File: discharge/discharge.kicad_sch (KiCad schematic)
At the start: 8 parts, among them J1 Conn_SDC, J2 Conn_HV_IN, J3 Conn_HV_OUT, J4 GND, J5 Conn_HV_IN, J6 Conn_HV_OUT, K1 Relay_SPST-NC, K2 Relay_SPST-NC

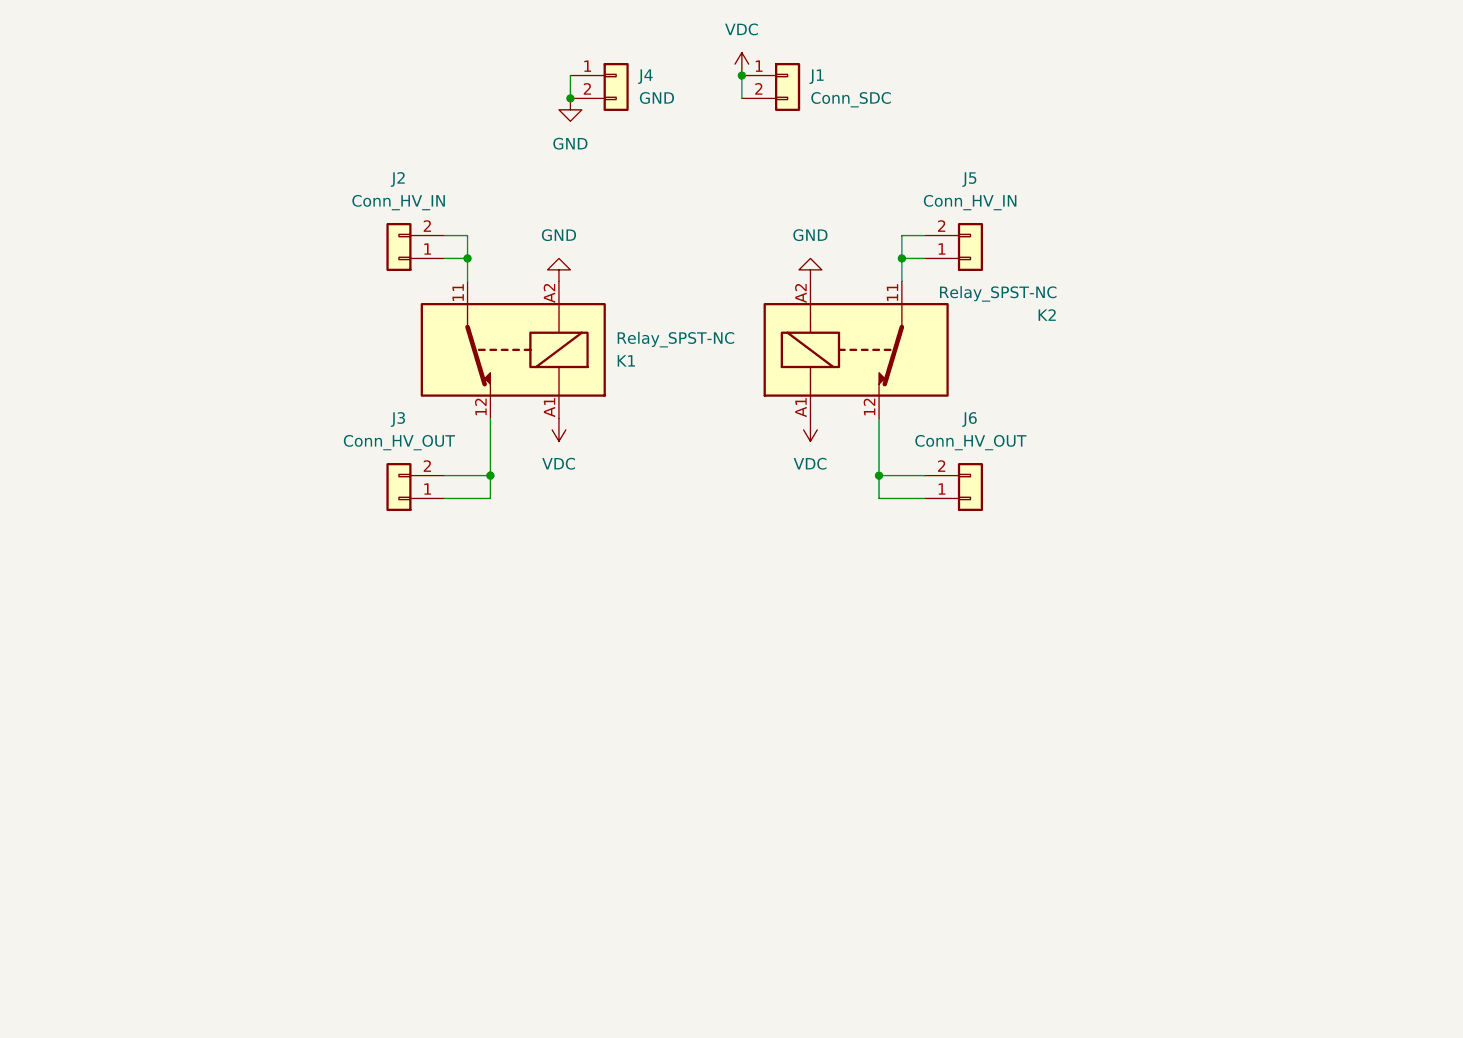
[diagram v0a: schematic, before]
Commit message: add timer
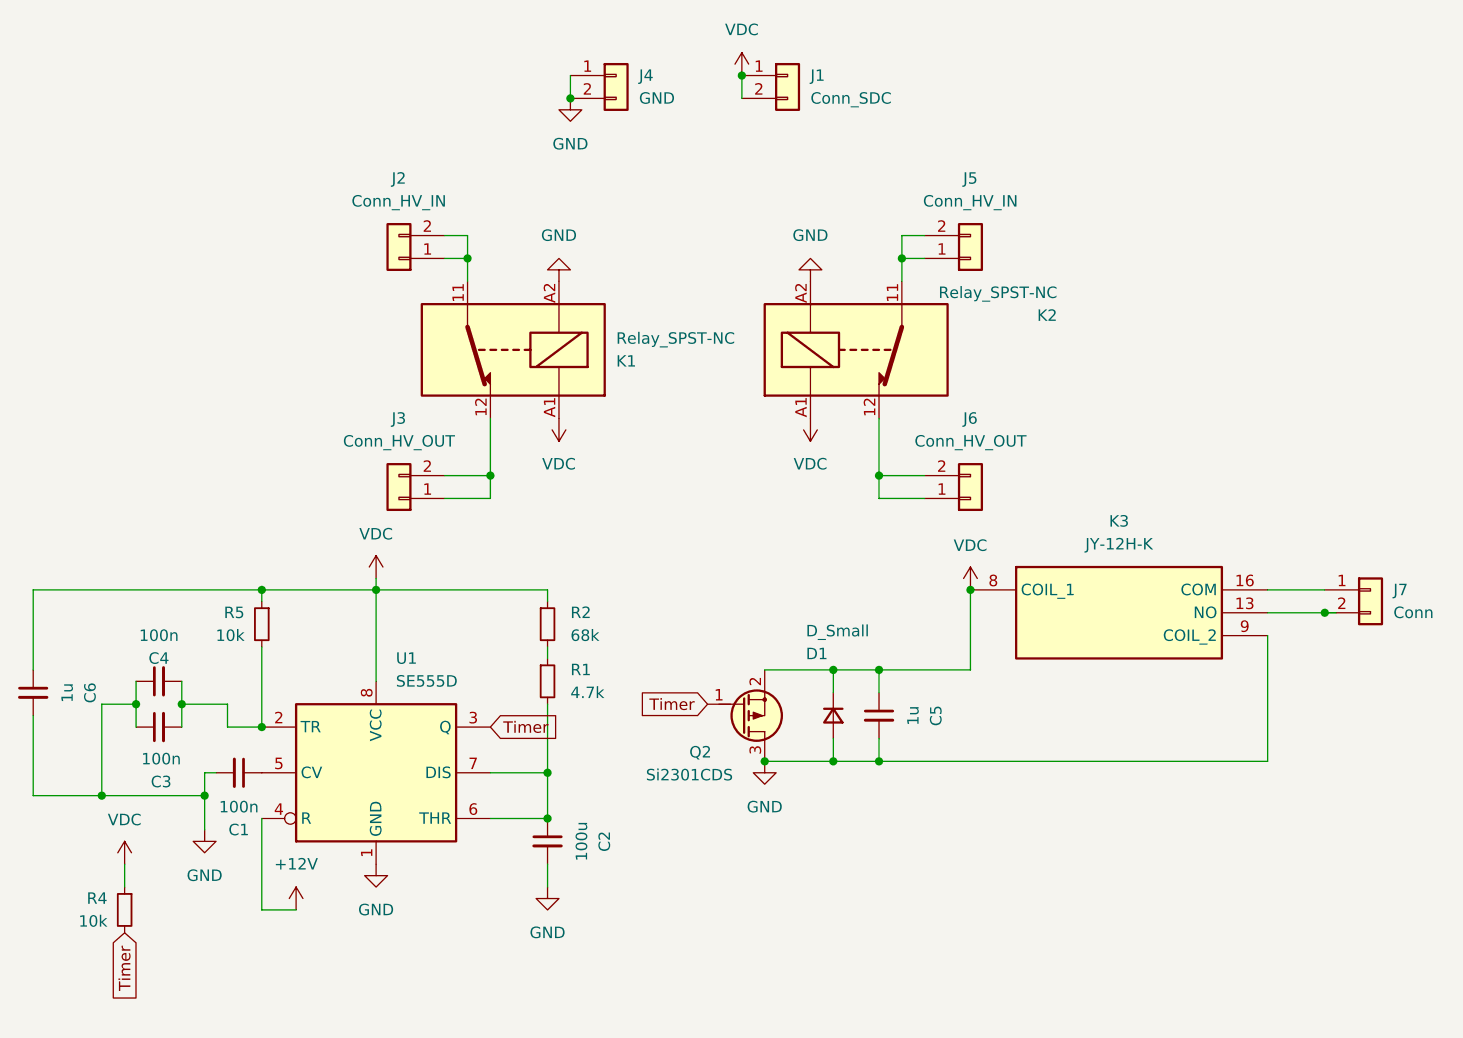
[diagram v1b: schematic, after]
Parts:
- added C1, C3, C4: 100n, Capacitor_SMD:C_0603_1608Metric, symbol Device:C_Small
- added C2: 100u, Capacitor_SMD:C_0603_1608Metric, symbol Device:C_Small
- added C5, C6: 1u, Capacitor_SMD:C_0603_1608Metric, symbol Device:C_Small
- added D1: D_Small, Diode_SMD:D_SOD-123F, symbol Device:D_Small
- added J7: Conn, Connector_JST:JST_XH_B2B-XH-A_1x02_P2.50mm_Vertical, symbol 178.6164.0001:Conn_01x02
- added K3: JY-12H-K, JY12HK, symbol JY-12H-K:JY-12H-K
- added Q2: Si2301CDS, Package_TO_SOT_SMD:SOT-23, symbol PCM_Transistor_MOSFET_AKL:Si2301CDS
- added R1: 4.7k, Resistor_SMD:R_0603_1608Metric, symbol Device:R_Small
- added R2: 68k, Resistor_SMD:R_0603_1608Metric, symbol Device:R_Small
- added R4, R5: 10k, Resistor_SMD:R_0603_1608Metric, symbol Device:R_Small
- added U1: SE555D, Package_SO:SOIC-8_3.9x4.9mm_P1.27mm, symbol Timer:SE555D
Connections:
- net GND: now also C1.2, C2.2, C3.1, C4.1, C5.2, C6.2, D1.2 (A), K3.9 (COIL_2), Q2.3 (D), U1.1 (GND)
- net VDC: now also C5.1, C6.1, D1.1 (K), K3.8 (COIL_1), Q2.2 (S), R2.1, R4.1, R5.1, U1.8 (VCC)
- new net: R1.1, R2.2
- new net: C3.2, C4.2, R5.2, U1.2 (TR)
- new net: J7.1 (Pin_1), K3.16 (COM)
- new net: J7.2 (Pin_2), K3.13 (NO)
- new net: C1.1, U1.5 (CV)
- new net: C2.1, R1.2, U1.6 (THR), U1.7 (DIS)
- new net +12V: U1.4 (R)
- new net Timer: Q2.1 (G), R4.2, U1.3 (Q)
